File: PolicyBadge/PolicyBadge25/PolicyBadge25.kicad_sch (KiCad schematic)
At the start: 10 parts, among them CN1 PH2.0-2P-LT, J1 Feed Point 915MHz, J4 Feed Point 2.4 GHz, SW3 TA-3525-A1, U1 MOUDLE-SEEEDUINO-XIAO-ESP32S3

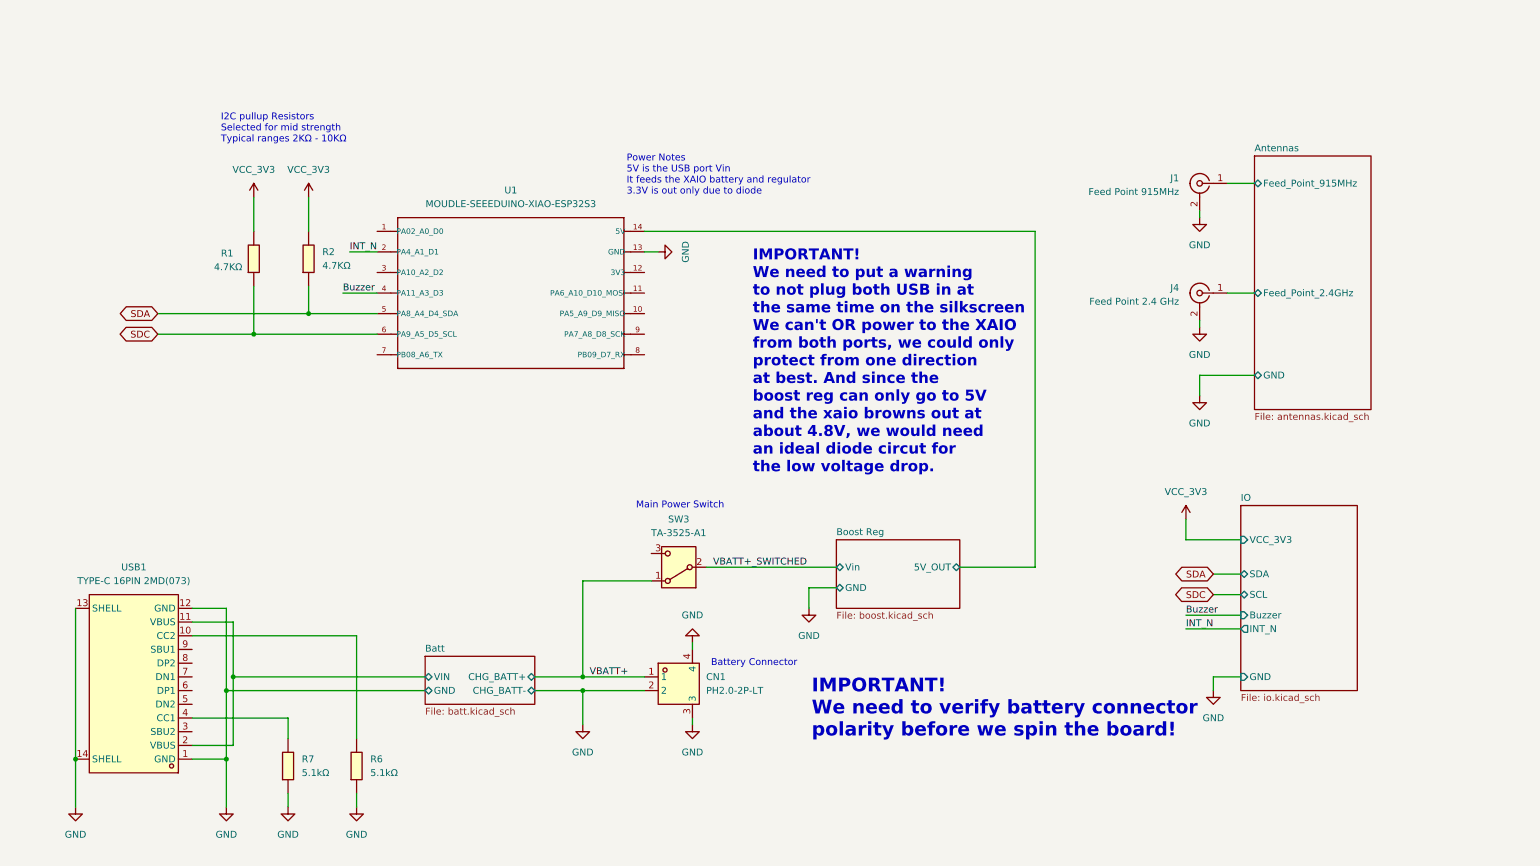
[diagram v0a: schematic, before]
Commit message: Released version of PCB
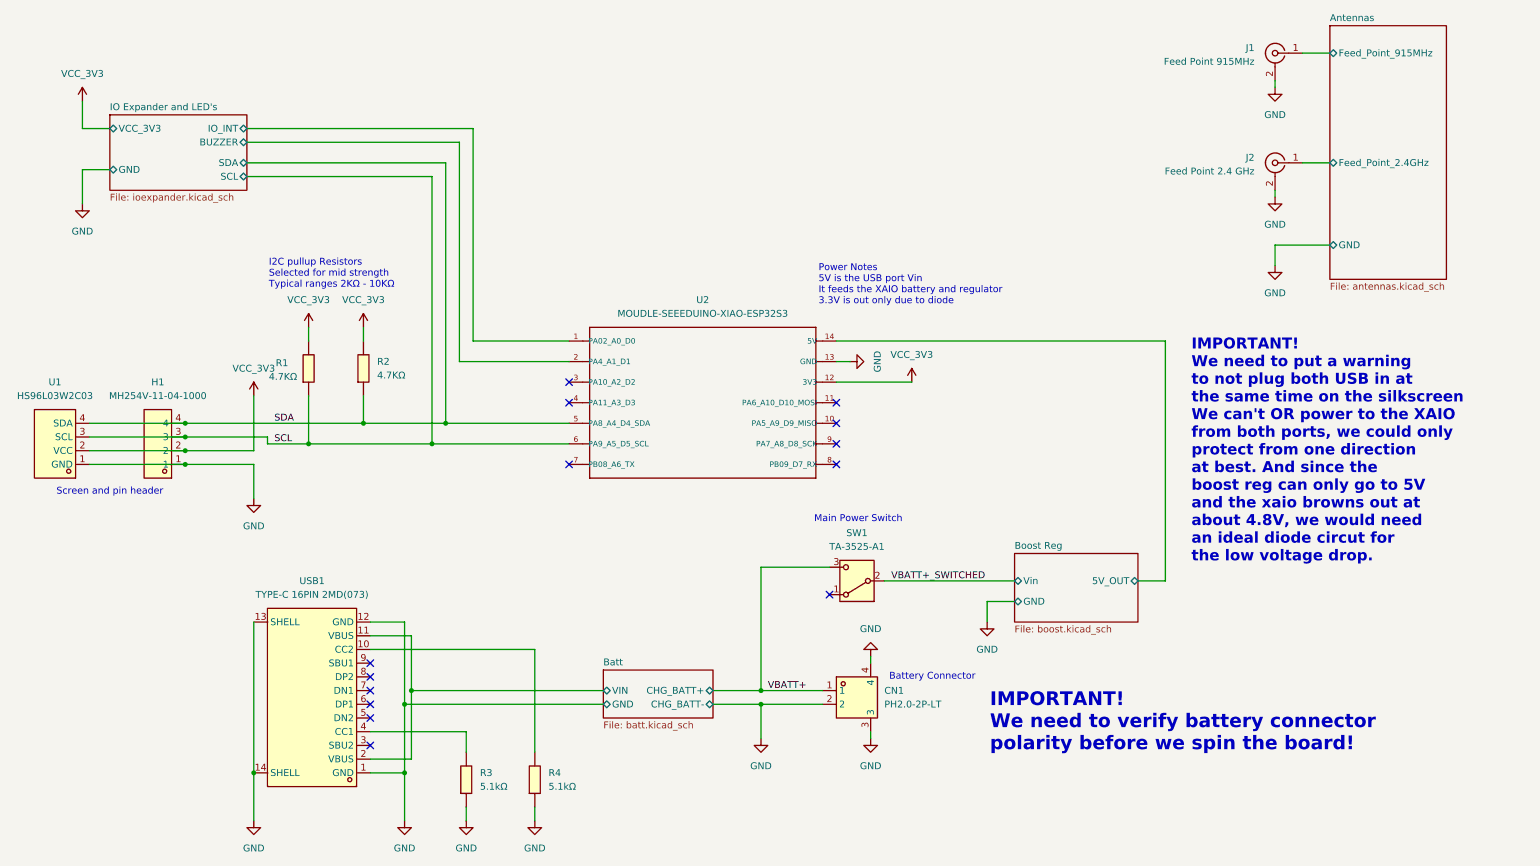
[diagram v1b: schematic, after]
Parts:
- added H1: MH254V-11-04-1000, imported:HDR-TH_4P-P2.54-V-M-3, symbol JLCPCB:MH254V-11-04-1000
- added U1: HS96L03W2C03, imported:OLED-TH_L27.8-W27.2-P2.54_C9900033791, symbol JLCPCB:HS96L03W2C03
- U2: renamed from U1; footprint MOUDLE14P-SMD-2.54-21X17.8MM -> XAIO ESP32S3:MOUDLE14P-SMD-2.54-21X17.8MM-header
- renumbered J4 to J2, R7 to R3, R6 to R4, SW3 to SW1
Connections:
- net GND: now also H1.1, U1.1 (GND)
- net SDA: now also H1.4, U1.4 (SDA)
- net VBATT+: now also SW1.3 (C); no longer SW1.1 (A)
- net VCC_3V3: now also U2.12 (3V3), H1.2, U1.2 (VCC)
- net IO Expander and LED's/IO_INT: now reaches U2.1 (PA02_A0_D0)
- net Buzzer: no longer names the net of U2.4 (PA11_A3_D3)
- net INT_N renamed IO Expander and LED's/BUZZER
- net SDC renamed SCL
- net SCL: now also H1.3, U1.3 (SCL)
- no-connect marks 0 -> 14
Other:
- removed sheet IO
- added sheet IO Expander and LED's (ioexpander.kicad_sch)
- note added: "Screen and pin header"
- moved on the sheet: CN1, J1, J2, R1, R2, R3, R4, SW1, U2, USB1
